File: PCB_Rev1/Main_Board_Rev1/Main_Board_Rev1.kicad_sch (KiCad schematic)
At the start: 2 parts, among them J1 Raspberry_Pi_2_3

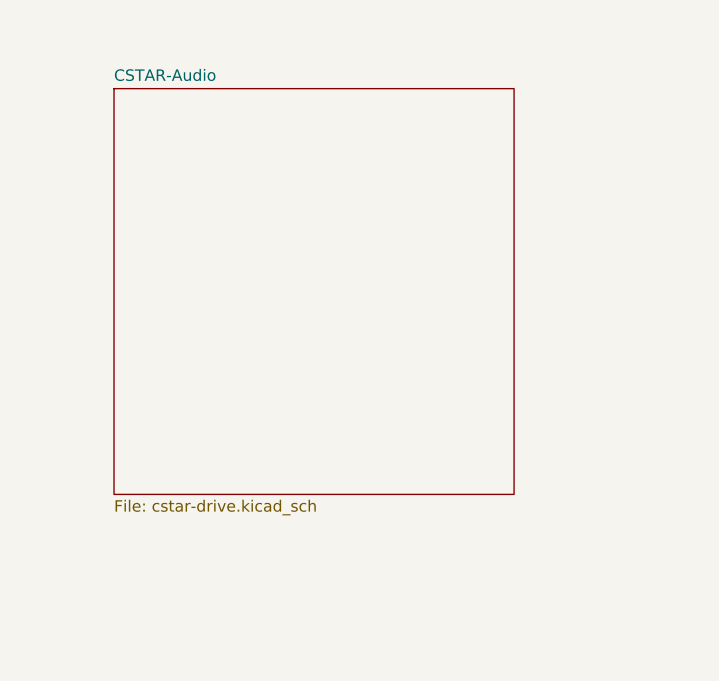
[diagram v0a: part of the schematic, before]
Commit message: Revert "Audio subsystem re-created"
This reverts commit 6dc47edf88eae56b01440ce5f2dfd5da155ce597.
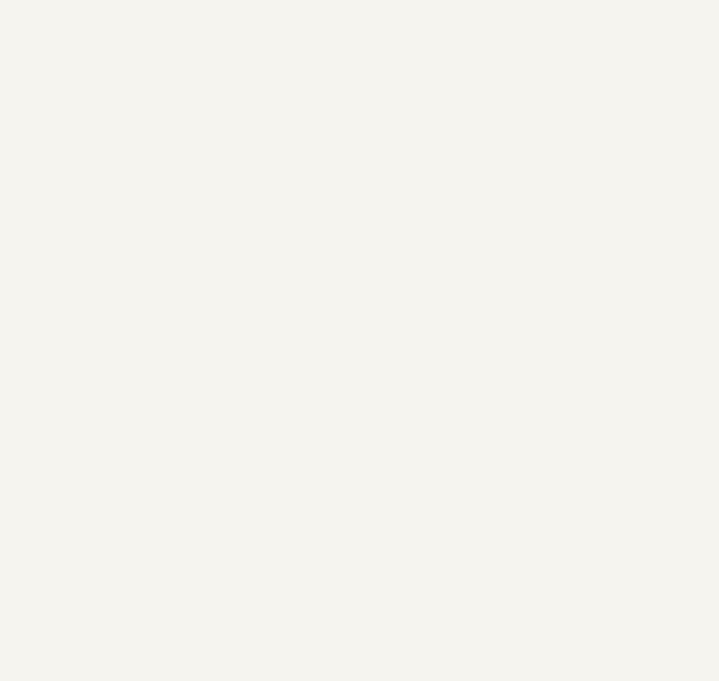
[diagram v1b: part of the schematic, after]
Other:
- removed sheet CSTAR-Audio
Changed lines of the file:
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@@
-		)
-	)
-	(sheet
-		(at 27.94 35.56)
-		(size 44.45 45.085)
-		(fields_autoplaced yes)
-		(stroke
-			(width 0.1524)
-			(type solid)
-		)
-		(fill
-			(color 0 0 0 0.0000)
-		)
-		(property "Sheetname" "CSTAR-Audio"
-			(at 27.94 34.8484 0)
-			(effects
-				(font
-					(size 1.27 1.27)
-				)
-				(justify left bottom)
-			)
-		)
-		(property "Sheetfile" "cstar-drive.kicad_sch"
-			(at 27.94 81.2296 0)
-			(effects
-				(font
-					(size 1.27 1.27)
-				)
-				(justify left top)
-			)
-		)
-		(instances
-			(project "Main_Board_Rev1"
-				(path "/8f5a23de-a1fa-4202-92fb-c2ac3de0338c"
-					(page "4")
-				)
-			)
 		)
 	)
